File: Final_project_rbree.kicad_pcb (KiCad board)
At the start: 2 copper layers, 99.7 x 99.7 mm, 48 parts, among them J1 Conn_01x02_Pin, J2 Conn_01x02_Pin, Q1 MMBT3904, Q3 AO3401A, U1 TL431, U2 LTV-817, U3 B1212, U4 2N7002, U7 NE555

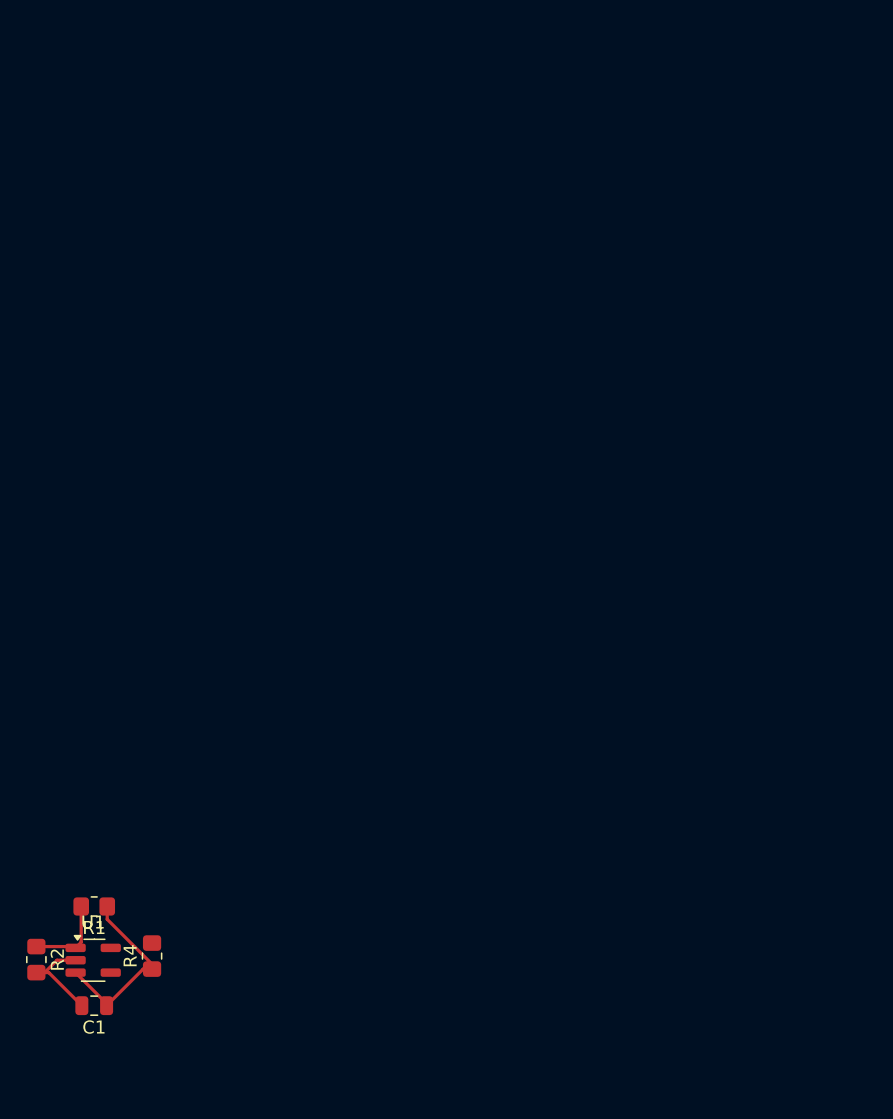
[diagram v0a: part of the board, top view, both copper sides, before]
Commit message: Update Final_project_rbree.kicad_pcb
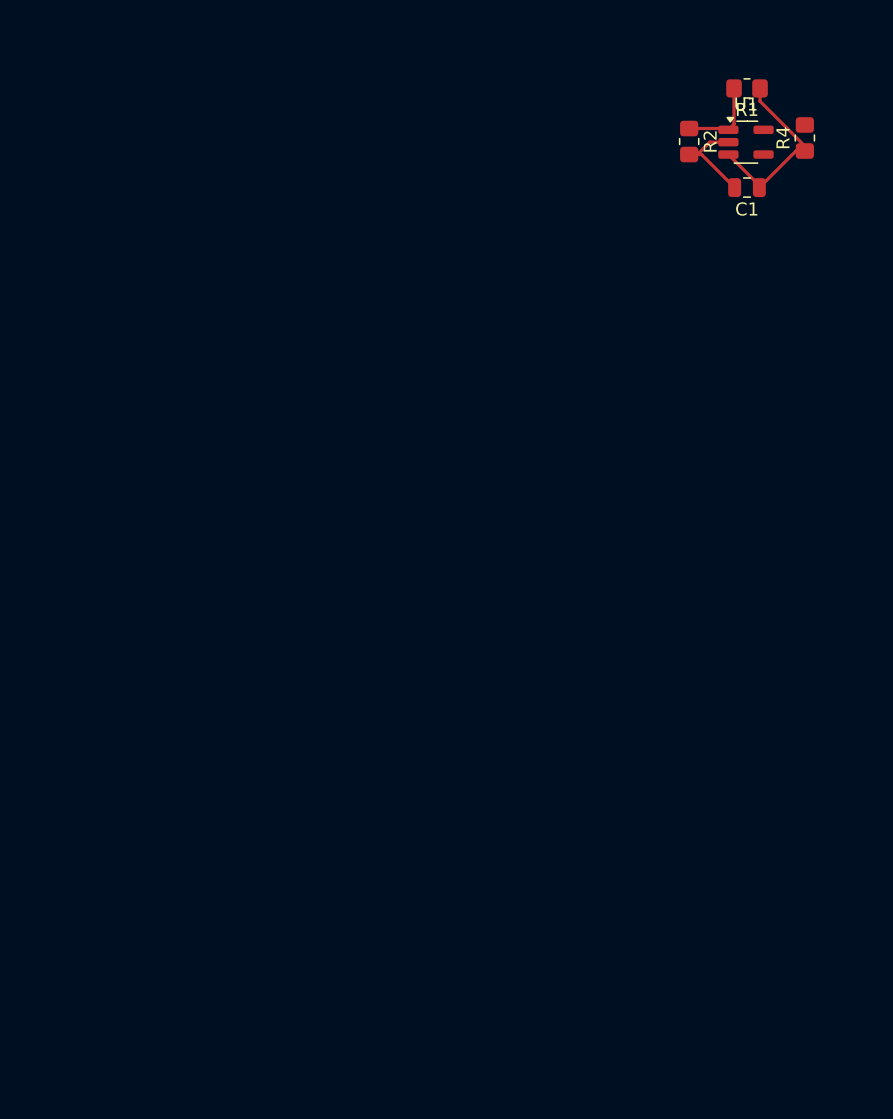
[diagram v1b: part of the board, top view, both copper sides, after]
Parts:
- moved U1 80.4 mm to (132.0, 55.6)
- moved C1 80.4 mm to (132.1, 59.1)
- moved R1 80.4 mm to (132.1, 51.4)
- moved R2 80.4 mm to (127.6, 55.5)
- moved R4 80.4 mm to (136.5, 55.2)
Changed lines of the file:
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@@
 		(tags "SOT-23-5 hand-soldering")
 		(property "Reference" "U4"
-			(at 0 -2.9 360)
+			(at 0 -2.9 0)
 			(layer "F.SilkS")
 			(effects
@@
 		)
 		(property "Value" "2N7002"
-			(at 0 2.9 360)
+			(at 0 2.9 0)
 			(layer "F.Fab")
 			(effects
@@
 	(footprint "Package_TO_SOT_SMD:SOT-23-5_HandSoldering"
 		(layer "F.Cu")
-		(at 81.835 118.43)
+		(at 132 55.565)
 		(descr "5-pin SOT23 package")
 		(tags "SOT-23-5 hand-soldering")
@@
 		(tags "THT DIP DIL PDIP 2.54mm 7.62mm 300mil SMDSocket SmallPads")
 		(property "Reference" "U2"
-			(at 0 -3.6 360)
+			(at 0 -3.6 0)
 			(layer "F.SilkS")
 			(effects
@@
 		)
 		(property "Value" "LTV-817"
-			(at 0 3.6 360)
+			(at 0 3.6 0)
 			(layer "F.Fab")
 			(effects
@@
 		)
 		(fp_text user "${REFERENCE}"
-			(at 0 0 360)
+			(at 0 0 0)
 			(layer "F.Fab")
 			(effects
@@
 		(tags "SOT TO_SOT_SMD")
 		(property "Reference" "Q1"
-			(at 0 -2.4 360)
+			(at 0 -2.4 0)
 			(layer "F.SilkS")
 			(effects
@@
 		)
 		(property "Value" "MMBT3904"
-			(at 0.3025 3.175 360)
+			(at 0.3025 3.175 0)
 			(layer "F.Fab")
 			(effects
@@
 		)
 		(fp_text user "${REFERENCE}"
-			(at 0 0 360)
+			(at 0 0 0)
 			(layer "F.Fab")
 			(effects
@@
 		(tags "resistor handsolder")
 		(property "Reference" "R12"
-			(at 0 -1.65 360)
+			(at 0 -1.65 0)
 			(layer "F.SilkS")
 			(effects
@@
 		)
 		(property "Value" "1M"
-			(at 0 1.65 360)
+			(at 0 1.65 0)
 			(layer "F.Fab")
 			(effects
@@
 		)
 		(fp_text user "${REFERENCE}"
-			(at 0.635 0 360)
+			(at 0.635 0 0)
 			(layer "F.Fab")
 			(effects
@@
 	(footprint "Resistor_SMD:R_0805_2012Metric_Pad1.20x1.40mm_HandSolder"
 		(layer "F.Cu")
-		(at 77.47 118.38 -90)
+		(at 127.635 55.515 -90)
 		(descr "Resistor SMD 0805 (2012 Metric), square (rectangular) end terminal, IPC_7351 nominal with elongated pad for handsoldering. (Body size source: IPC-SM-782 page 72, https://www.pcb-3d.com/wordpress/wp-content/uploads/ipc-sm-782a_amendment_1_and_2.pdf), generated with kicad-footprint-generator")
 		(tags "resistor handsolder")
@@
 		(tags "resistor handsolder")
 		(property "Reference" "R16"
-			(at -1 -3.175 360)
+			(at -1 -3.175 0)
 			(layer "F.SilkS")
 			(effects
@@
 		)
 		(property "Value" "22k"
-			(at 0 1.65 360)
+			(at 0 1.65 0)
 			(layer "F.Fab")
 			(effects
@@
 		)
 		(fp_text user "${REFERENCE}"
-			(at 0 0 360)
+			(at 0 0 0)
 			(layer "F.Fab")
 			(effects
@@
 		(tags "connector JST VH vertical")
 		(property "Reference" "Conn_01x1"
-			(at 9.9 -4.9 360)
+			(at 9.9 -4.9 0)
 			(layer "F.SilkS")
 			(effects
@@
 		)
 		(property "Value" "Conn_01x06"
-			(at 9.9 6 360)
+			(at 9.9 6 0)
 			(layer "F.Fab")
 			(effects
@@
 		)
 		(fp_text user "${REFERENCE}"
-			(at 9.9 4.1 360)
+			(at 9.9 4.1 0)
 			(layer "F.Fab")
 			(effects
@@
 		(tags "resistor handsolder")
 		(property "Reference" "R13"
-			(at 0 -1.65 360)
+			(at 0 -1.65 0)
 			(layer "F.SilkS")
 			(effects
@@
 		)
 		(property "Value" "2k2"
-			(at 0 1.65 360)
+			(at 0 1.65 0)
 			(layer "F.Fab")
 			(effects
@@
 		(tags "Diode DO-35_SOD27 series Axial Horizontal pin pitch 7.62mm  length 4mm diameter 2mm")
 		(property "Reference" "D1"
-			(at 3.81 -2.12 360)
+			(at 3.81 -2.12 0)
 			(layer "F.SilkS")
 			(effects
@@
 		)
 		(property "Value" "12V"
-			(at 3.81 2.12 360)
+			(at 3.81 2.12 0)
 			(layer "F.Fab")
 			(effects
@@
 		)
 		(fp_text user "K"
-			(at 0 -1.8 360)
+			(at 0 -1.8 0)
 			(layer "F.SilkS")
 			(effects
@@
 		)
 		(fp_text user "K"
-			(at 0 -1.8 360)
+			(at 0 -1.8 0)
 			(layer "F.Fab")
 			(effects
@@
 		)
 		(fp_text user "${REFERENCE}"
-			(at 4.11 0 360)
+			(at 4.11 0 0)
 			(layer "F.Fab")
 			(effects
@@
 		(tags "resistor handsolder")
 		(property "Reference" "R19"
-			(at 0 -1.65 360)
+			(at 0 -1.65 0)
 			(layer "F.SilkS")
 			(effects
@@
 		)
 		(fp_text user "${REFERENCE}"
-			(at 0 0 360)
+			(at 0 0 0)
 			(layer "F.Fab")
 			(effects
@@
 	(footprint "Resistor_SMD:R_0805_2012Metric_Pad1.20x1.40mm_HandSolder"
 		(layer "F.Cu")
-		(at 86.36 118.11 90)
+		(at 136.525 55.245 90)
 		(descr "Resistor SMD 0805 (2012 Metric), square (rectangular) end terminal, IPC_7351 nominal with elongated pad for handsoldering. (Body size source: IPC-SM-782 page 72, https://www.pcb-3d.com/wordpress/wp-content/uploads/ipc-sm-782a_amendment_1_and_2.pdf), generated with kicad-footprint-generator")
 		(tags "resistor handsolder")
@@
 		(tags "resistor handsolder")
 		(property "Reference" "R15"
-			(at 0 -1.65 360)
+			(at 0 -1.65 0)
 			(layer "F.SilkS")
 			(effects
@@
 		)
 		(property "Value" "22k"
-			(at 0 1.65 360)
+			(at 0 1.65 0)
 			(layer "F.Fab")
 			(effects
@@
 		)
 		(fp_text user "${REFERENCE}"
-			(at 0 0 360)
+			(at 0 0 0)
 			(layer "F.Fab")
 			(effects
@@
 	(footprint "Capacitor_SMD:C_0805_2012Metric"
 		(layer "F.Cu")
-		(at 81.915 121.92 180)
+		(at 132.08 59.055 180)
 		(descr "Capacitor SMD 0805 (2012 Metric), square (rectangular) end terminal, IPC_7351 nominal, (Body size source: IPC-SM-782 page 76, https://www.pcb-3d.com/wordpress/wp-content/uploads/ipc-sm-782a_amendment_1_and_2.pdf, https://docs.google.com/spreadsheets/d/1BsfQQcO9C6DZCsRaXUlFlo91Tg2WpOkGARC1WS5S8t0/edit?usp=sharing), generated with kicad-footprint-generator")
 		(tags "capacitor")
 		(property "Reference" "C1"
-			(at 0 -1.68 360)
+			(at 0 -1.68 0)
 			(layer "F.SilkS")
 			(effects
@@
 		)
 		(property "Value" "0.1uF"
-			(at 0 1.68 360)
+			(at 0 1.68 0)
 			(layer "F.Fab")
 			(effects
@@
 		)
 		(fp_text user "${REFERENCE}"
-			(at 0 0 360)
+			(at 0 0 0)
 			(layer "F.Fab")
 			(effects
@@
 	(footprint "Resistor_SMD:R_0805_2012Metric_Pad1.20x1.40mm_HandSolder"
 		(layer "F.Cu")
-		(at 81.915 114.3 180)
+		(at 132.08 51.435 180)
 		(descr "Resistor SMD 0805 (2012 Metric), square (rectangular) end terminal, IPC_7351 nominal with elongated pad for handsoldering. (Body size source: IPC-SM-782 page 72, https://www.pcb-3d.com/wordpress/wp-content/uploads/ipc-sm-782a_amendment_1_and_2.pdf), generated with kicad-footprint-generator")
 		(tags "resistor handsolder")
 		(property "Reference" "R1"
-			(at 0 -1.65 360)
+			(at 0 -1.65 0)
 			(layer "F.SilkS")
 			(effects
@@
 		)
 		(property "Value" "2k"
-			(at 0 1.65 360)
+			(at 0 1.65 0)
 			(layer "F.Fab")
 			(effects
@@
 		)
 		(fp_text user "${REFERENCE}"
-			(at 0 0 360)
+			(at 0 0 0)
 			(layer "F.Fab")
 			(effects
@@
 	)
 	(segment
-		(start 77.47 119.38)
-		(end 78.105 119.38)
+		(start 127.635 56.515)
+		(end 128.27 56.515)
 		(width 0.25)
 		(layer "F.Cu")
@@
 	)
 	(segment
-		(start 79.055 118.43)
-		(end 80.485 118.43)
+		(start 129.22 55.565)
+		(end 130.65 55.565)
 		(width 0.25)
 		(layer "F.Cu")
@@
 	)
 	(segment
-		(start 78.425 119.38)
-		(end 80.965 121.92)
+		(start 128.59 56.515)
+		(end 131.13 59.055)
 		(width 0.25)
 		(layer "F.Cu")
@@
 	)
 	(segment
-		(start 78.105 119.38)
-		(end 79.055 118.43)
+		(start 128.27 56.515)
+		(end 129.22 55.565)
 		(width 0.25)
 		(layer "F.Cu")
@@
 	)
 	(segment
-		(start 77.47 119.38)
-		(end 78.425 119.38)
+		(start 127.635 56.515)
+		(end 128.59 56.515)
 		(width 0.25)
 		(layer "F.Cu")
@@
 	)
 	(segment
-		(start 85.675 119.11)
-		(end 86.36 119.11)
+		(start 135.84 56.245)
+		(end 136.525 56.245)
 		(width 0.25)
 		(layer "F.Cu")
@@
 	)
 	(segment
-		(start 80.485 119.38)
-		(end 82.865 121.76)
+		(start 130.65 56.515)
+		(end 133.03 58.895)
 		(width 0.25)
 		(layer "F.Cu")
@@
 	)
 	(segment
-		(start 82.865 121.76)
-		(end 82.865 121.92)
+		(start 133.03 58.895)
+		(end 133.03 59.055)
 		(width 0.25)
 		(layer "F.Cu")
@@
 	)
 	(segment
-		(start 82.865 121.92)
-		(end 85.675 119.11)
+		(start 133.03 59.055)
+		(end 135.84 56.245)
 		(width 0.25)
 		(layer "F.Cu")
@@
 	)
 	(segment
-		(start 82.915 115.2851)
-		(end 86.36 118.7301)
+		(start 133.08 52.4201)
+		(end 136.525 55.8651)
 		(width 0.25)
 		(layer "F.Cu")
@@
 	)
 	(segment
-		(start 82.915 114.3)
-		(end 82.915 115.2851)
+		(start 133.08 51.435)
+		(end 133.08 52.4201)
 		(width 0.25)
 		(layer "F.Cu")
@@
 	)
 	(segment
-		(start 86.36 118.7301)
-		(end 86.36 119.11)
+		(start 136.525 55.8651)
+		(end 136.525 56.245)
 		(width 0.25)
 		(layer "F.Cu")
@@
 	)
 	(segment
-		(start 80.385 117.38)
-		(end 80.485 117.48)
+		(start 130.55 54.515)
+		(end 130.65 54.615)
 		(width 0.25)
 		(layer "F.Cu")
@@
 	)
 	(segment
-		(start 80.915 114.3)
-		(end 80.915 117.05)
+		(start 131.08 51.435)
+		(end 131.08 54.185)
 		(width 0.25)
 		(layer "F.Cu")
@@
 	)
 	(segment
-		(start 77.47 117.38)
-		(end 80.385 117.38)
+		(start 127.635 54.515)
+		(end 130.55 54.515)
 		(width 0.25)
 		(layer "F.Cu")
@@
 	)
 	(segment
-		(start 80.915 117.05)
-		(end 80.485 117.48)
+		(start 131.08 54.185)
+		(end 130.65 54.615)
 		(width 0.25)
 		(layer "F.Cu")

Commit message: commit - final
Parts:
- removed the REF** at (181.0, 37.5)
- removed the REF** at (271.1, 127.0)
- removed the REF** at (180.3, 127.0)
- added R22: 1k, Resistor_SMD:R_0805_2012Metric_Pad1.20x1.40mm_HandSolder, F.Cu at (223.2, 77.5)
- added R23: 1k, Resistor_SMD:R_0805_2012Metric_Pad1.20x1.40mm_HandSolder, F.Cu at (220.3, 81.9)
- added REF**: MountingHole_3.2mm_M3_ISO7380, MountingHole:MountingHole_3.2mm_M3_ISO7380, F.Cu at (-3.69, -93.7)
- added REF**: MountingHole_3.2mm_M3_ISO7380, MountingHole:MountingHole_3.2mm_M3_ISO7380, F.Cu at (186.0, 35.5)
- added REF**: MountingHole_3.2mm_M3_ISO7380, MountingHole:MountingHole_3.2mm_M3_ISO7380, F.Cu at (185.3, 125.1)
- added REF**: MountingHole_3.2mm_M3_ISO7380, MountingHole:MountingHole_3.2mm_M3_ISO7380, F.Cu at (276.2, 125.1)
- U7: footprint Package_SO:SOIC-8-1EP_3.9x4.9mm_P1.27mm_EP2.29x3mm -> Package_SO:SOIC-8_3.9x4.9mm_P1.27mm
- moved R14 173.6 mm to (252.9, 74.9)
- moved C4 71.1 mm to (240.3, 46.4), turned to 180 degrees
- moved D2 42.8 mm to (275.5, 78.2)
- moved Q3 38.9 mm to (251.1, 112.1), turned to 0 degrees
- moved D3 38.4 mm to (245.7, 103.5), turned to -90 degrees
- moved R19 33.1 mm to (251.4, 104.1), turned to 180 degrees
- moved R21 31.5 mm to (251.4, 107.9), turned to 180 degrees
- moved R20 29.2 mm to (251.4, 100.6), turned to 0 degrees
- moved U4 29.0 mm to (248.2, 78.7), turned to 0 degrees
- moved R13 26.9 mm to (217.5, 51.4)
- moved R9 26.7 mm to (196.8, 79.4), turned to 180 degrees
- moved Q1 24.6 mm to (247.2, 94.3), turned to 0 degrees
- moved U1 22.7 mm to (154.2, 50.8)
- moved R2 22.7 mm to (149.9, 50.7)
- moved C1 22.7 mm to (154.3, 54.3)
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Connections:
- C1 pad 1: /Vref -> (no net)
- R1 pad 1: /Vref -> (no net)
- R4 pad 1: /Vref -> (no net)
- U1 pad 3: /Vref -> (no net)
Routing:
- net VCC: track 19.8 -> 171.3 mm
- net GLV+: track 8.42 -> 50.7 mm
- net (no net): track 0.00 -> 14.4 mm
- net /Vref: track 14.4 -> 0.00 mm
- net /RED+: track 0.00 -> 13.7 mm
- net Net-(J1-Pin_2): track 11.8 -> 0.00 mm
- net GLV-: track 11.5 -> 0.00 mm
- net Net-(U4-G): track 0.00 -> 10.8 mm
- net Net-(U7-THR): track 6.75 -> 14.5 mm
- net Net-(Q1-B): track 0.00 -> 6.56 mm
- net Net-(U7-DIS): track 6.30 -> 12.5 mm
- net Net-(Q1-C): track 13.3 -> 19.5 mm
- net Net-(U4-D): track 6.04 -> 11.8 mm
- net +12V: track 8.94 -> 3.70 mm
- net Net-(U7-Q): track 2.35 -> 6.86 mm
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- added copper zone on B.Cu, net GLV-
- added copper zone on F.Cu, net GLV-
